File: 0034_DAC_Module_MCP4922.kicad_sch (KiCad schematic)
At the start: 7 parts, among them J1 Screw_Terminal_01x02, J2 Screw_Terminal_01x02, U1 MCP4922-ESL

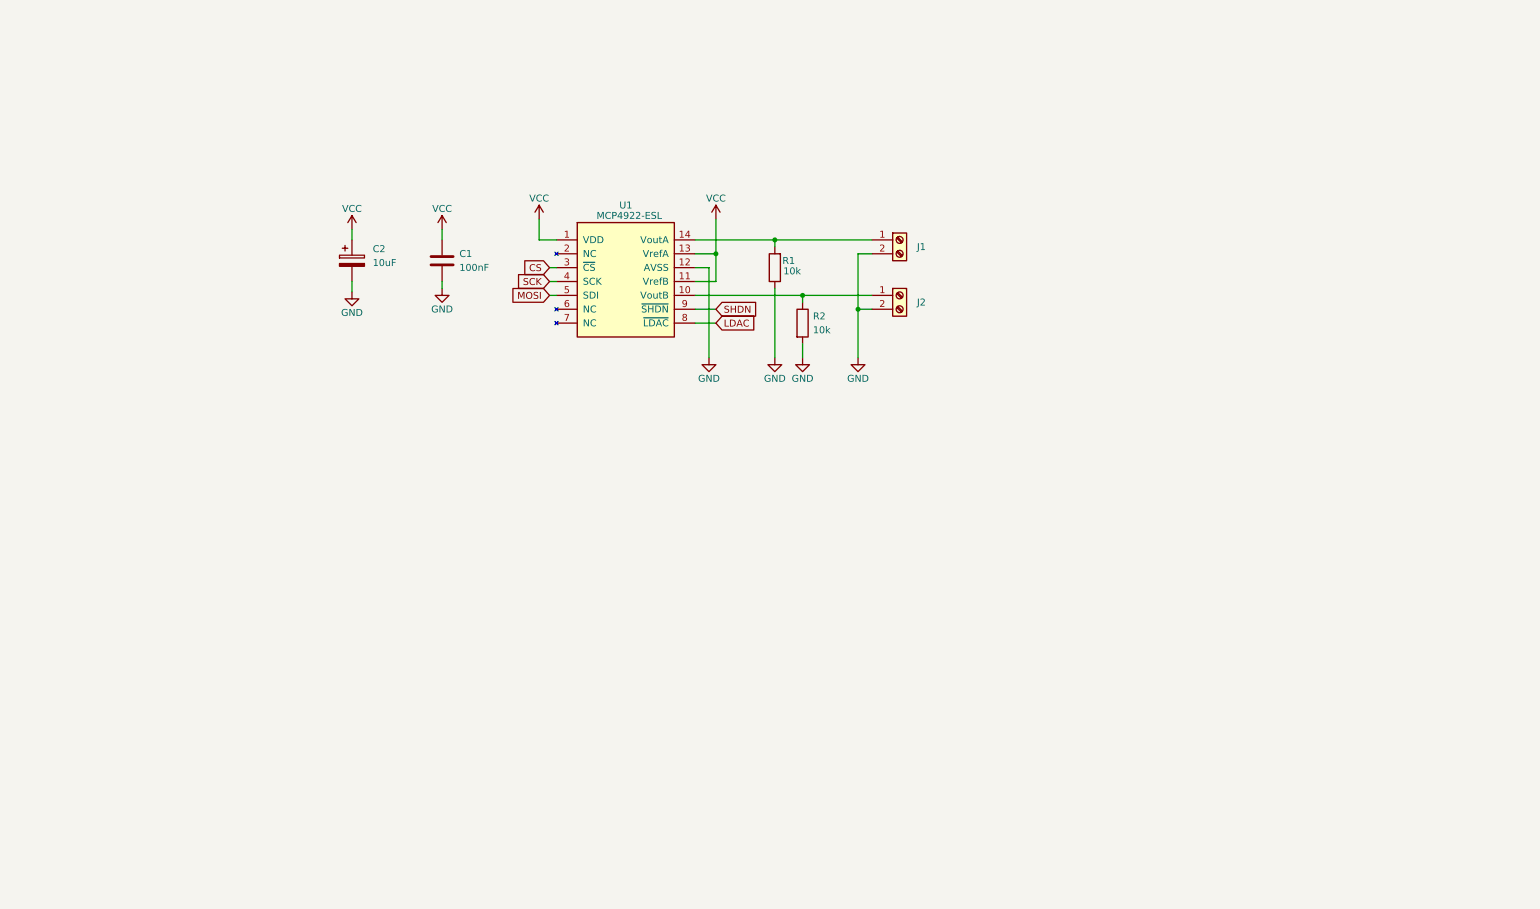
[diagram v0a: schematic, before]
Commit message: Add files via upload
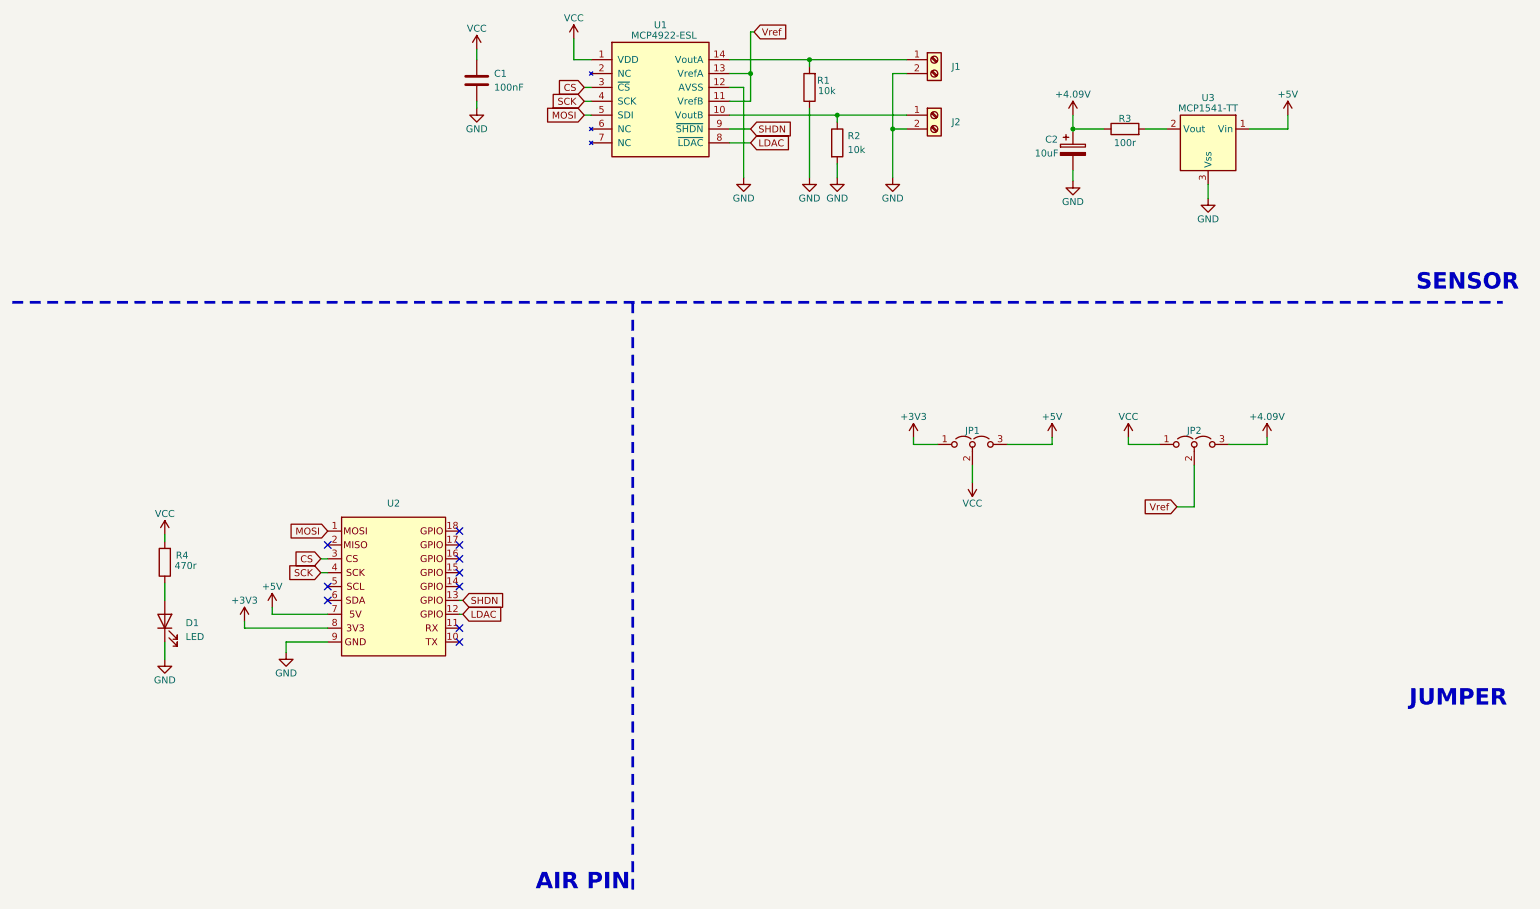
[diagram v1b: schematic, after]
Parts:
- added D1: LED, LED_SMD:LED_0805_2012Metric, symbol Device:LED
- added JP1, JP2: Jumper_3_Open, Jumper:SolderJumper-3_P1.3mm_Open_Pad1.0x1.5mm, symbol Jumper:Jumper_3_Open
- added R3: 100r, Resistor_SMD:R_0805_2012Metric, symbol Device:R
- added R4: 470r, Resistor_SMD:R_0805_2012Metric, symbol Device:R
- added U2: ~, Moduler_:pin_header, symbol moduler_pin:air
- added U3: MCP1541-TT, Package_TO_SOT_SMD:SOT-23, symbol Reference_Voltage:MCP1541-TT
- C1: footprint (none) -> Capacitor_SMD:C_0805_2012Metric
- C2: footprint (none) -> Capacitor_Tantalum_SMD:CP_EIA-3216-10_Kemet-I
- J1, J2: footprint (none) -> Connector_PinHeader_2.54mm:PinHeader_1x02_P2.54mm_Vertical
- R1, R2: footprint (none) -> Resistor_SMD:R_0805_2012Metric
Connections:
- net CS: now also U2.3
- net GND: now also D1.1 (K), U2.9, U3.3 (Vss)
- net LDAC: now also U2.12
- net MOSI: now also U2.1
- net SCK: now also U2.4
- net SHDN: now also U2.13
- net VCC: now also JP1.2 (C), JP2.1 (A), R4.2; no longer C2.1, U1.11 (VrefB), U1.13 (VrefA)
- new net: R3.2, U3.2 (Vout)
- new net: D1.2 (A), R4.1
- new net +3V3: JP1.1 (A), U2.8
- new net +4V: C2.1, JP2.3 (B), R3.1
- new net +5V: JP1.3 (B), U2.7, U3.1 (Vin)
- new net Vref: JP2.2 (C), U1.11 (VrefB), U1.13 (VrefA)
- no-connect marks 0 -> 10
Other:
- note added: "AIR PIN"
- note added: "JUMPER"
- note added: "SENSOR"
- moved on the sheet: C1, J1, J2, R1, R2, U1
